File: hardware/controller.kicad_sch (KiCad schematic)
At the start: 41 parts, among them J1 Connector, USB-TYPE-C-16P, J2 AXK6F20347YG, J3 AFA01-S08FCA-00, U1 ESP32-C6-WROOM-1, U2 BQ24074RGTR, U3 TLA2518IRTER, U6 TPS62142RGTR

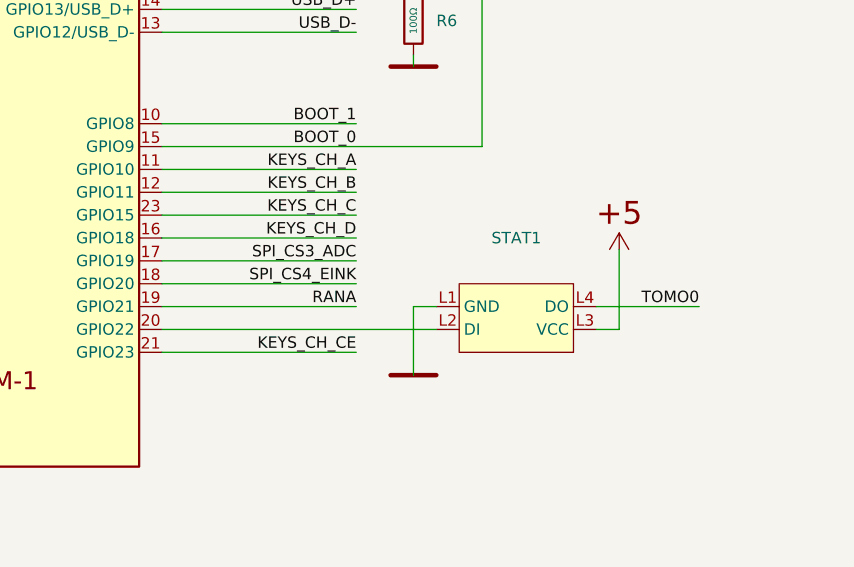
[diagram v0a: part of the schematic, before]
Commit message: :sparkles: finish all hardware designs
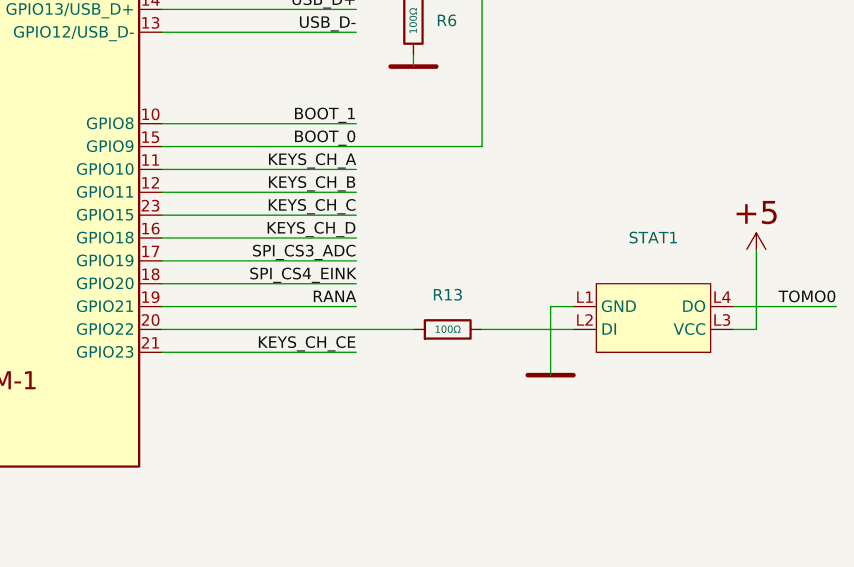
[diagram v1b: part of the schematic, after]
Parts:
- added R13: 100Ω, KeysDock:R_0402, symbol components:0402,100Ω
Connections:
- net at STAT1.L2 (DI): now also R13.2; no longer U1.20 (GPIO22)
- new net: R13.1, U1.20 (GPIO22)
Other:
- moved on the sheet: STAT1
